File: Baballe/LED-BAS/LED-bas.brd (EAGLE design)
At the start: 30 x 32 mm, 15 parts, among them Q1 200mA/50V, Q2 200mA/50V, Q3 200mA/50V

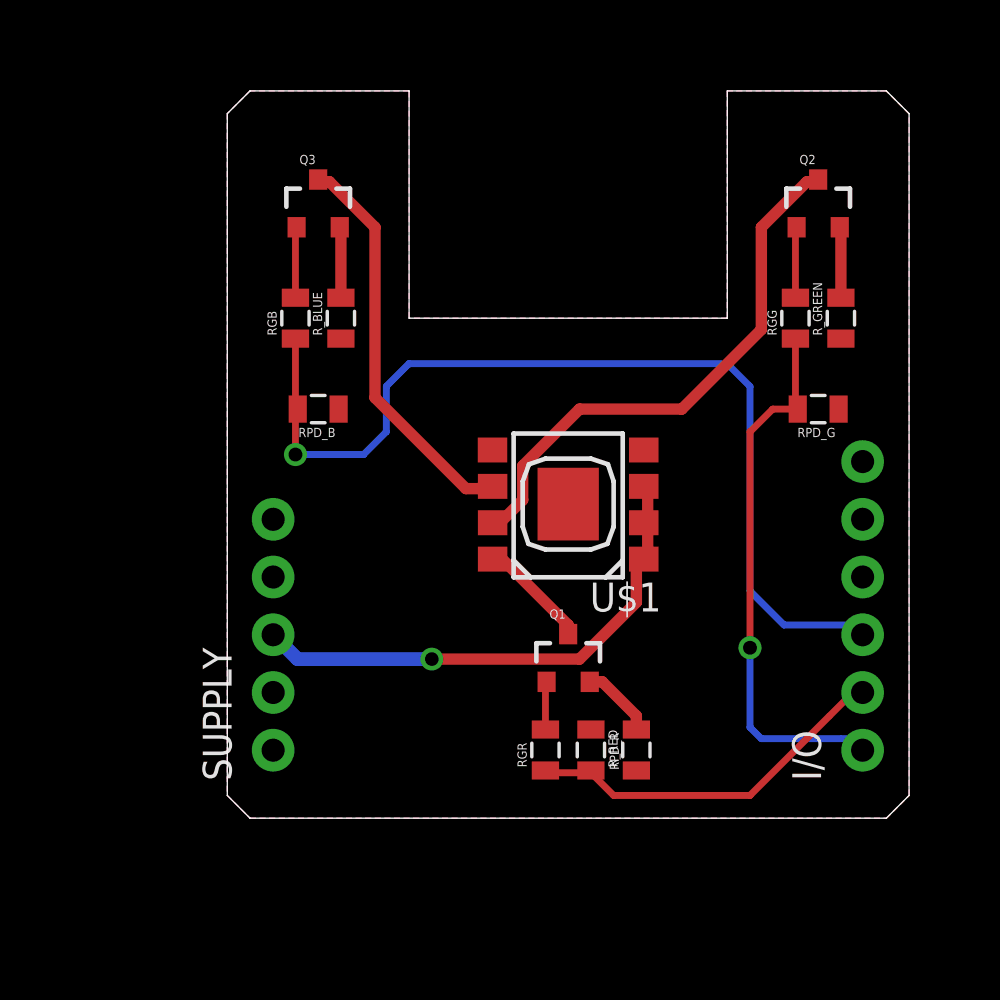
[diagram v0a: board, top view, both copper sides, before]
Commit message: V2 de la Baballe
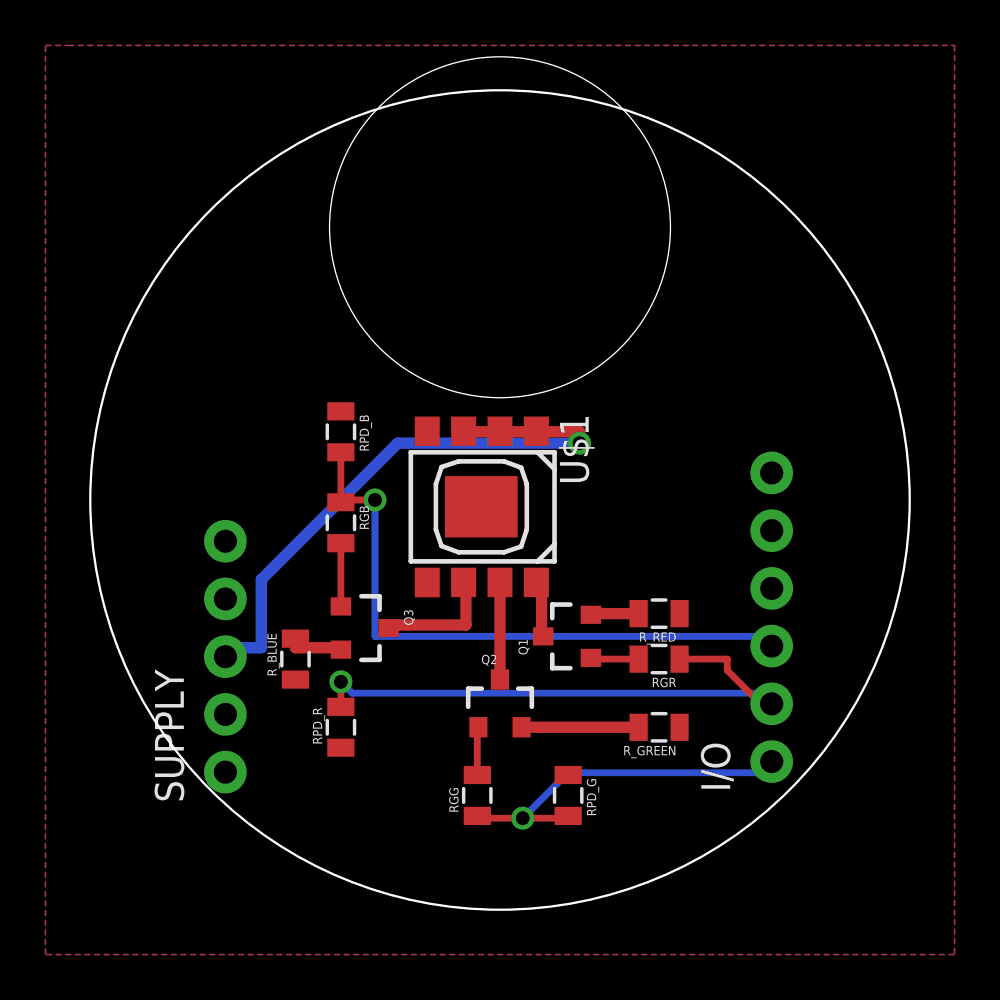
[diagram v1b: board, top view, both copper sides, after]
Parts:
- moved Q2 26.1 mm to (56.0, 5.00)
- moved RGG 25.2 mm to (55.0, 1.00)
- moved RPD_G 20.2 mm to (59.0, 1.00), turned to 270 degrees
- moved R_GREEN 19.7 mm to (63.0, 4.00), turned to 180 degrees
- moved Q3 18.7 mm to (50.0, 8.37), turned to 270 degrees
- moved R_BLUE 15.1 mm to (47.0, 7.00)
- moved RPD_R 11.0 mm to (49.0, 4.00), turned to 90 degrees
- moved RGB 9.22 mm to (49.0, 13.0), turned to 270 degrees
- moved RGR 6.40 mm to (63.0, 7.00), turned to 180 degrees
- moved R_RED 6.08 mm to (63.0, 9.00), turned to 180 degrees
- moved I/O 4.03 mm to (68.0, 2.49)
- moved U$1 3.08 mm to (56.0, 13.7), turned to 270 degrees
- moved SUPPLY 2.31 mm to (43.9, 2.03)
- moved RPD_B 1.41 mm to (49.0, 17.0), turned to 270 degrees
- moved Q1 1.00 mm to (59.0, 8.00), turned to 90 degrees
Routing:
- net N$8: track 24.2 -> 4.28 mm
- net O_BLUE: track 43.2 -> 27.3 mm
- net N$9: track 17.8 -> 5.31 mm
- net O_RED: track 16.5 -> 25.6 mm, vias 0 -> 1
- net O_GREEN: track 24.4 -> 16.2 mm
- net V_IN: track 23.1 -> 27.0 mm
- net N$2: track 3.15 -> 5.15 mm
- net N$7: track 4.98 -> 3.04 mm
- net N$3: track 3.27 -> 2.15 mm
- net N$4: track 3.15 -> 2.15 mm
- net N$1: track 3.15 -> 2.58 mm
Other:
- board size 30 x 32 mm -> 36.1 x 36.1 mm
